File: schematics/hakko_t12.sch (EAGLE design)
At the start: 46 parts, among them IC1 ATMEGA328-20P, IC2 AD822, Q1 IRF9540, Q2 16MHZ, T1 2N2222, T2 2N2222, T3 2N2907

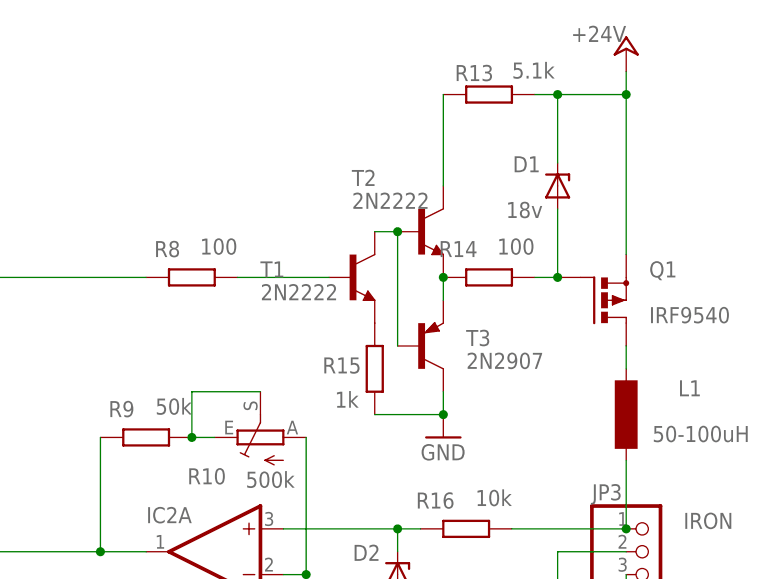
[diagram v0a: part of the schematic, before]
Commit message: Add files via upload
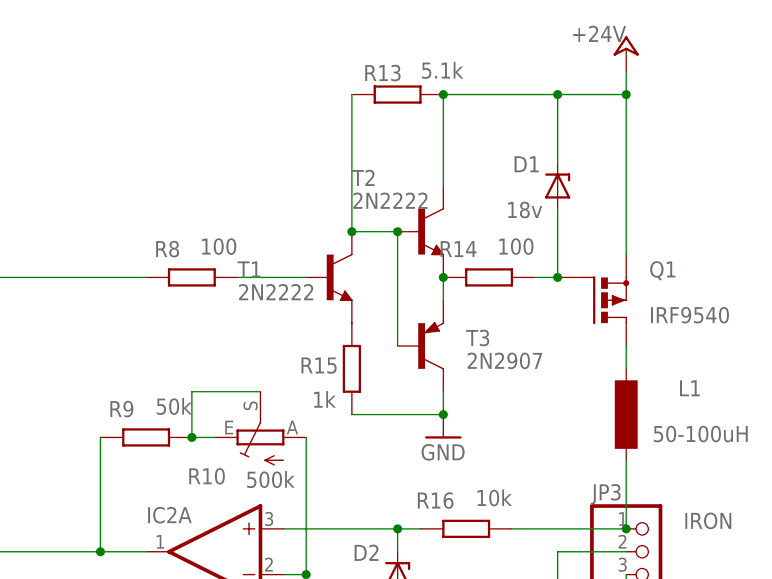
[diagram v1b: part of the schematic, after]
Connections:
- removed net N$37: R13.1, T2.C
- net +24V: now also T2.C
- net N$35: now also R13.1
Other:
- moved on the sheet: R13, R15, T1
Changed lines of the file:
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@@
 <?xml version="1.0" encoding="utf-8"?>
 <!DOCTYPE eagle SYSTEM "eagle.dtd">
-<eagle version="9.2.2">
+<eagle version="9.5.2">
 <drawing>
 <settings>
@@
 <attribute name="VALUE" x="257.556" y="105.41" size="1.778" layer="96" rot="R180"/>
 </instance>
-<instance part="T1" gate="G$1" x="213.36" y="121.92" smashed="yes">
-<attribute name="NAME" x="203.2" y="121.92" size="1.778" layer="95"/>
-<attribute name="VALUE" x="203.2" y="119.38" size="1.778" layer="96"/>
+<instance part="T1" gate="G$1" x="210.82" y="121.92" smashed="yes">
+<attribute name="NAME" x="200.66" y="121.92" size="1.778" layer="95"/>
+<attribute name="VALUE" x="200.66" y="119.38" size="1.778" layer="96"/>
 </instance>
 <instance part="T2" gate="G$1" x="220.98" y="127" smashed="yes">
@@
 <attribute name="VALUE" x="175.26" y="45.72" size="1.778" layer="96"/>
 </instance>
-<instance part="R15" gate="G$1" x="215.9" y="111.76" smashed="yes" rot="R90">
-<attribute name="NAME" x="214.4014" y="113.03" size="1.778" layer="95" rot="R180"/>
-<attribute name="VALUE" x="214.122" y="109.22" size="1.778" layer="96" rot="R180"/>
-</instance>
-<instance part="R13" gate="G$1" x="228.6" y="142.24" smashed="yes">
-<attribute name="NAME" x="224.79" y="143.7386" size="1.778" layer="95"/>
-<attribute name="VALUE" x="231.14" y="144.018" size="1.778" layer="96"/>
+<instance part="R15" gate="G$1" x="213.36" y="111.76" smashed="yes" rot="R90">
+<attribute name="NAME" x="211.8614" y="113.03" size="1.778" layer="95" rot="R180"/>
+<attribute name="VALUE" x="211.582" y="109.22" size="1.778" layer="96" rot="R180"/>
+</instance>
+<instance part="R13" gate="G$1" x="218.44" y="142.24" smashed="yes">
+<attribute name="NAME" x="214.63" y="143.7386" size="1.778" layer="95"/>
+<attribute name="VALUE" x="220.98" y="144.018" size="1.778" layer="96"/>
 </instance>
 <instance part="D1" gate="G$1" x="236.22" y="132.08" smashed="yes" rot="R90">
@@
 <wire x1="223.52" y1="106.68" x2="223.52" y2="109.22" width="0.1524" layer="91"/>
 <pinref part="R15" gate="G$1" pin="1"/>
-<wire x1="215.9" y1="106.68" x2="223.52" y2="106.68" width="0.1524" layer="91"/>
+<wire x1="213.36" y1="106.68" x2="223.52" y2="106.68" width="0.1524" layer="91"/>
 <junction x="223.52" y="106.68"/>
 </segment>
@@
 <wire x1="218.44" y1="114.3" x2="218.44" y2="127" width="0.1524" layer="91"/>
 <pinref part="T1" gate="G$1" pin="C"/>
-<wire x1="218.44" y1="127" x2="215.9" y2="127" width="0.1524" layer="91"/>
+<wire x1="218.44" y1="127" x2="213.36" y2="127" width="0.1524" layer="91"/>
 <junction x="218.44" y="127"/>
+<pinref part="R13" gate="G$1" pin="1"/>
+<wire x1="213.36" y1="127" x2="213.36" y2="142.24" width="0.1524" layer="91"/>
+<junction x="213.36" y="127"/>
 </segment>
 </net>
@@
 <pinref part="T1" gate="G$1" pin="E"/>
 <pinref part="R15" gate="G$1" pin="2"/>
-</segment>
-</net>
-<net name="N$37" class="0">
-<segment>
-<pinref part="T2" gate="G$1" pin="C"/>
-<pinref part="R13" gate="G$1" pin="1"/>
-<wire x1="223.52" y1="132.08" x2="223.52" y2="142.24" width="0.1524" layer="91"/>
 </segment>
 </net>
@@
 <wire x1="243.84" y1="124.46" x2="243.84" y2="142.24" width="0.1524" layer="91"/>
 <wire x1="243.84" y1="142.24" x2="236.22" y2="142.24" width="0.1524" layer="91"/>
-<pinref part="R13" gate="G$1" pin="2"/>
 <pinref part="P+2" gate="1" pin="+24V"/>
-<wire x1="236.22" y1="142.24" x2="233.68" y2="142.24" width="0.1524" layer="91"/>
 <wire x1="243.84" y1="142.24" x2="243.84" y2="144.78" width="0.1524" layer="91"/>
 <junction x="243.84" y="142.24"/>
 <pinref part="D1" gate="G$1" pin="C"/>
 <wire x1="236.22" y1="134.62" x2="236.22" y2="142.24" width="0.1524" layer="91"/>
+<pinref part="T2" gate="G$1" pin="C"/>
+<wire x1="223.52" y1="132.08" x2="223.52" y2="142.24" width="0.1524" layer="91"/>
+<wire x1="223.52" y1="142.24" x2="236.22" y2="142.24" width="0.1524" layer="91"/>
 <junction x="236.22" y="142.24"/>
+<pinref part="R13" gate="G$1" pin="2"/>
+<junction x="223.52" y="142.24"/>
 </segment>
 <segment>
@@
 <pinref part="T1" gate="G$1" pin="B"/>
 <pinref part="R8" gate="G$1" pin="2"/>
-<wire x1="210.82" y1="121.92" x2="200.66" y2="121.92" width="0.1524" layer="91"/>
-</segment>
-</net>
+<wire x1="208.28" y1="121.92" x2="200.66" y2="121.92" width="0.1524" layer="91"/>
+</segment>
+</net>

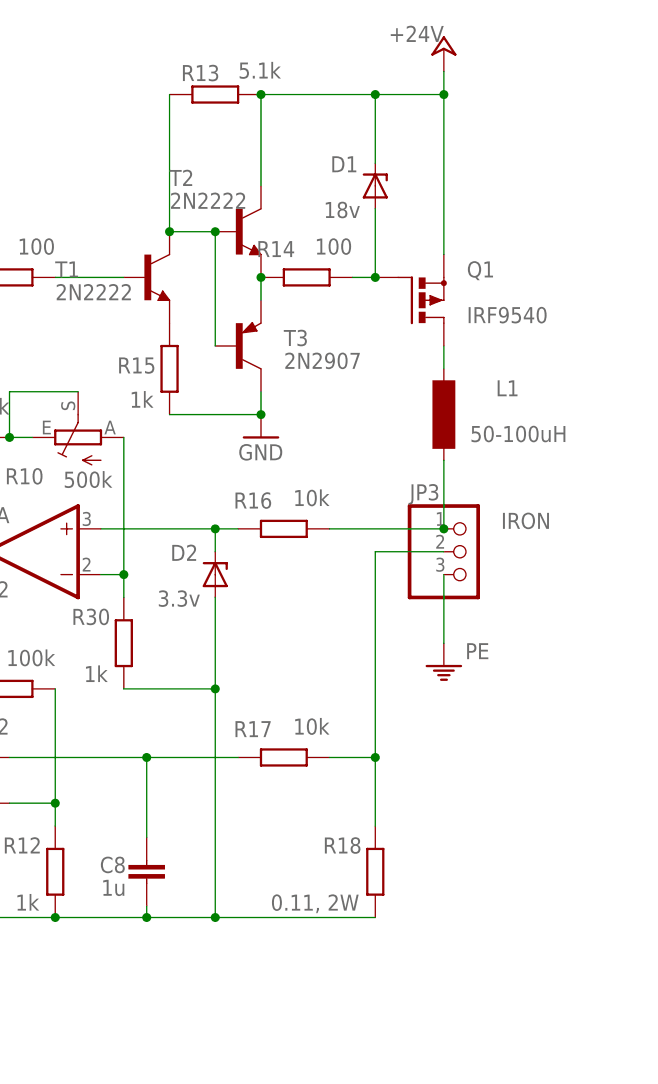
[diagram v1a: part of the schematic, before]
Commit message: Add files via upload
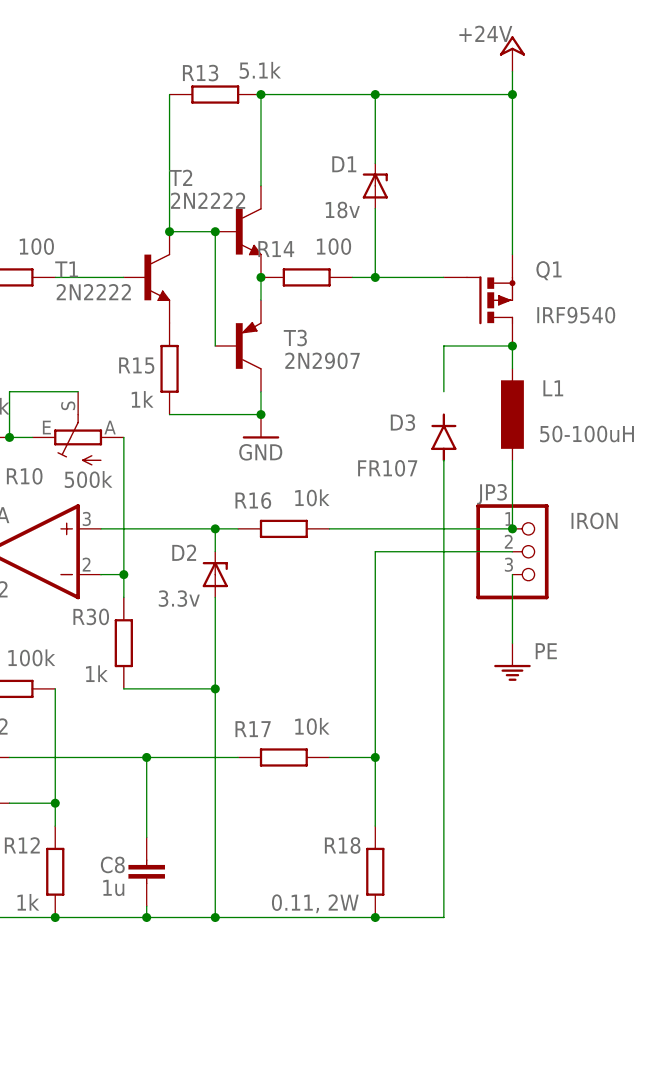
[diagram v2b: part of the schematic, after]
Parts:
- added D3: FR107, diode:1N4004
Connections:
- net GND: now also D3.A
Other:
- moved on the sheet: JP3, L1, Q1
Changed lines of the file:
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@@
 <?xml version="1.0" encoding="utf-8"?>
 <!DOCTYPE eagle SYSTEM "eagle.dtd">
-<eagle version="9.5.2">
+<eagle version="9.6.1">
 <drawing>
 <settings>
@@
 <layer number="97" name="Info" color="7" fill="1" visible="yes" active="yes"/>
 <layer number="98" name="Guide" color="6" fill="1" visible="yes" active="yes"/>
+<layer number="99" name="SpiceOrder" color="5" fill="1" visible="yes" active="yes"/>
 <layer number="100" name="Muster" color="7" fill="1" visible="no" active="no"/>
 <layer number="101" name="Patch_Top" color="12" fill="4" visible="yes" active="yes"/>
@@
 <part name="PE1" library="supply1" library_urn="urn:adsk.eagle:library:371" deviceset="PE" device=""/>
 <part name="GND7" library="supply1" library_urn="urn:adsk.eagle:library:371" deviceset="GND" device=""/>
+<part name="D3" library="diode" library_urn="urn:adsk.eagle:library:210" deviceset="1N4004" device="" package3d_urn="urn:adsk.eagle:package:43336/1" value="FR107"/>
 </parts>
 <sheets>
@@
 <attribute name="VALUE" x="54.61" y="115.57" size="1.778" layer="96" rot="R180"/>
 </instance>
-<instance part="P+2" gate="1" x="243.84" y="147.32" smashed="yes">
-<attribute name="VALUE" x="243.84" y="149.86" size="1.778" layer="96" rot="R180"/>
+<instance part="P+2" gate="1" x="251.46" y="147.32" smashed="yes">
+<attribute name="VALUE" x="251.46" y="149.86" size="1.778" layer="96" rot="R180"/>
 </instance>
 <instance part="GND1" gate="1" x="41.91" y="41.91" smashed="yes">
@@
 <attribute name="VALUE" x="113.03" y="106.68" size="1.778" layer="96" rot="R180"/>
 </instance>
-<instance part="L1" gate="G$1" x="243.84" y="106.68" smashed="yes" rot="R90">
-<attribute name="NAME" x="252.222" y="110.49" size="1.778" layer="95" rot="R180"/>
-<attribute name="VALUE" x="257.556" y="105.41" size="1.778" layer="96" rot="R180"/>
+<instance part="L1" gate="G$1" x="251.46" y="106.68" smashed="yes" rot="R90">
+<attribute name="NAME" x="257.302" y="110.49" size="1.778" layer="95" rot="R180"/>
+<attribute name="VALUE" x="265.176" y="105.41" size="1.778" layer="96" rot="R180"/>
 </instance>
 <instance part="T1" gate="G$1" x="210.82" y="121.92" smashed="yes">
@@
 <attribute name="VALUE" x="233.68" y="126.238" size="1.778" layer="96" rot="R180"/>
 </instance>
-<instance part="Q1" gate="G$1" x="241.3" y="119.38" smashed="yes">
-<attribute name="NAME" x="246.38" y="121.92" size="1.778" layer="95"/>
-<attribute name="VALUE" x="246.38" y="116.84" size="1.778" layer="96"/>
+<instance part="Q1" gate="G$1" x="248.92" y="119.38" smashed="yes">
+<attribute name="NAME" x="254" y="121.92" size="1.778" layer="95"/>
+<attribute name="VALUE" x="254" y="116.84" size="1.778" layer="96"/>
 </instance>
 <instance part="GND9" gate="1" x="223.52" y="104.14" smashed="yes">
@@
 <attribute name="VALUE" x="120.65" y="120.65" size="1.778" layer="96"/>
 </instance>
-<instance part="JP3" gate="A" x="246.38" y="91.44" smashed="yes">
-<attribute name="NAME" x="240.03" y="97.155" size="1.778" layer="95"/>
-<attribute name="VALUE" x="250.19" y="93.98" size="1.778" layer="96"/>
-</instance>
-<instance part="PE1" gate="M" x="243.84" y="78.74" smashed="yes">
-<attribute name="VALUE" x="248.92" y="81.28" size="1.778" layer="96" rot="R180"/>
+<instance part="JP3" gate="A" x="254" y="91.44" smashed="yes">
+<attribute name="NAME" x="247.65" y="97.155" size="1.778" layer="95"/>
+<attribute name="VALUE" x="257.81" y="93.98" size="1.778" layer="96"/>
+</instance>
+<instance part="PE1" gate="M" x="251.46" y="78.74" smashed="yes">
+<attribute name="VALUE" x="256.54" y="81.28" size="1.778" layer="96" rot="R180"/>
 </instance>
 <instance part="GND7" gate="1" x="88.9" y="96.52" smashed="yes">
 <attribute name="VALUE" x="86.36" y="93.98" size="1.778" layer="96"/>
+</instance>
+<instance part="D3" gate="1" x="243.84" y="104.14" smashed="yes" rot="R90">
+<attribute name="NAME" x="240.8174" y="106.68" size="1.778" layer="95" rot="R180"/>
+<attribute name="VALUE" x="241.0714" y="101.6" size="1.778" layer="96" rot="R180"/>
 </instance>
 </instances>
@@
 <pinref part="GND5" gate="1" pin="GND"/>
 <junction x="177.8" y="50.8"/>
+<pinref part="D3" gate="1" pin="A"/>
+<wire x1="243.84" y1="101.6" x2="243.84" y2="50.8" width="0.1524" layer="91"/>
+<wire x1="243.84" y1="50.8" x2="236.22" y2="50.8" width="0.1524" layer="91"/>
+<junction x="236.22" y="50.8"/>
 </segment>
 <segment>
@@
 <pinref part="L1" gate="G$1" pin="2"/>
 <pinref part="Q1" gate="G$1" pin="D"/>
-<wire x1="243.84" y1="111.76" x2="243.84" y2="114.3" width="0.1524" layer="91"/>
+<wire x1="251.46" y1="111.76" x2="251.46" y2="114.3" width="0.1524" layer="91"/>
+<wire x1="243.84" y1="109.22" x2="243.84" y2="114.3" width="0.1524" layer="91"/>
+<wire x1="243.84" y1="114.3" x2="251.46" y2="114.3" width="0.1524" layer="91"/>
+<junction x="251.46" y="114.3"/>
 </segment>
 </net>
@@
 <pinref part="Q1" gate="G$1" pin="G"/>
 <pinref part="R14" gate="G$1" pin="2"/>
+<wire x1="243.84" y1="121.92" x2="236.22" y2="121.92" width="0.1524" layer="91"/>
 <pinref part="D1" gate="G$1" pin="A"/>
-<wire x1="236.22" y1="121.92" x2="236.22" y2="129.54" width="0.1524" layer="91"/>
+<wire x1="236.22" y1="121.92" x2="233.68" y2="121.92" width="0.1524" layer="91"/>
+<wire x1="236.22" y1="129.54" x2="236.22" y2="121.92" width="0.1524" layer="91"/>
 <junction x="236.22" y="121.92"/>
-<wire x1="236.22" y1="121.92" x2="233.68" y2="121.92" width="0.1524" layer="91"/>
 </segment>
 </net>
@@
 <junction x="218.44" y="127"/>
 <pinref part="R13" gate="G$1" pin="1"/>
-<wire x1="213.36" y1="127" x2="213.36" y2="142.24" width="0.1524" layer="91"/>
+<wire x1="213.36" y1="142.24" x2="213.36" y2="127" width="0.1524" layer="91"/>
 <junction x="213.36" y="127"/>
 </segment>
@@
 <segment>
 <pinref part="Q1" gate="G$1" pin="S"/>
-<wire x1="243.84" y1="124.46" x2="243.84" y2="142.24" width="0.1524" layer="91"/>
-<wire x1="243.84" y1="142.24" x2="236.22" y2="142.24" width="0.1524" layer="91"/>
+<wire x1="251.46" y1="124.46" x2="251.46" y2="142.24" width="0.1524" layer="91"/>
+<wire x1="251.46" y1="142.24" x2="236.22" y2="142.24" width="0.1524" layer="91"/>
 <pinref part="P+2" gate="1" pin="+24V"/>
-<wire x1="243.84" y1="142.24" x2="243.84" y2="144.78" width="0.1524" layer="91"/>
-<junction x="243.84" y="142.24"/>
+<wire x1="251.46" y1="142.24" x2="251.46" y2="144.78" width="0.1524" layer="91"/>
+<junction x="251.46" y="142.24"/>
 <pinref part="D1" gate="G$1" pin="C"/>
 <wire x1="236.22" y1="134.62" x2="236.22" y2="142.24" width="0.1524" layer="91"/>
 <pinref part="T2" gate="G$1" pin="C"/>
+<pinref part="R13" gate="G$1" pin="2"/>
 <wire x1="223.52" y1="132.08" x2="223.52" y2="142.24" width="0.1524" layer="91"/>
 <wire x1="223.52" y1="142.24" x2="236.22" y2="142.24" width="0.1524" layer="91"/>
+<junction x="223.52" y="142.24"/>
 <junction x="236.22" y="142.24"/>
-<pinref part="R13" gate="G$1" pin="2"/>
-<junction x="223.52" y="142.24"/>
 </segment>
 <segment>
@@
 <pinref part="L1" gate="G$1" pin="1"/>
 <pinref part="JP3" gate="A" pin="1"/>
-<wire x1="243.84" y1="101.6" x2="243.84" y2="93.98" width="0.1524" layer="91"/>
+<wire x1="251.46" y1="101.6" x2="251.46" y2="93.98" width="0.1524" layer="91"/>
 <pinref part="R16" gate="G$1" pin="2"/>
-<wire x1="243.84" y1="93.98" x2="231.14" y2="93.98" width="0.1524" layer="91"/>
-<junction x="243.84" y="93.98"/>
+<wire x1="251.46" y1="93.98" x2="231.14" y2="93.98" width="0.1524" layer="91"/>
+<junction x="251.46" y="93.98"/>
 </segment>
 </net>
@@
 <segment>
 <pinref part="JP3" gate="A" pin="2"/>
-<wire x1="236.22" y1="91.44" x2="243.84" y2="91.44" width="0.1524" layer="91"/>
+<wire x1="236.22" y1="91.44" x2="251.46" y2="91.44" width="0.1524" layer="91"/>
 <pinref part="R18" gate="G$1" pin="2"/>
 <wire x1="236.22" y1="60.96" x2="236.22" y2="68.58" width="0.1524" layer="91"/>
@@
 <pinref part="PE1" gate="M" pin="PE"/>
 <pinref part="JP3" gate="A" pin="3"/>
-<wire x1="243.84" y1="81.28" x2="243.84" y2="88.9" width="0.1524" layer="91"/>
-</segment>
-</net>
+<wire x1="251.46" y1="81.28" x2="251.46" y2="88.9" width="0.1524" layer="91"/>
+</segment>
+</net>
